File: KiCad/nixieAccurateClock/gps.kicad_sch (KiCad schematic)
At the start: 3 parts

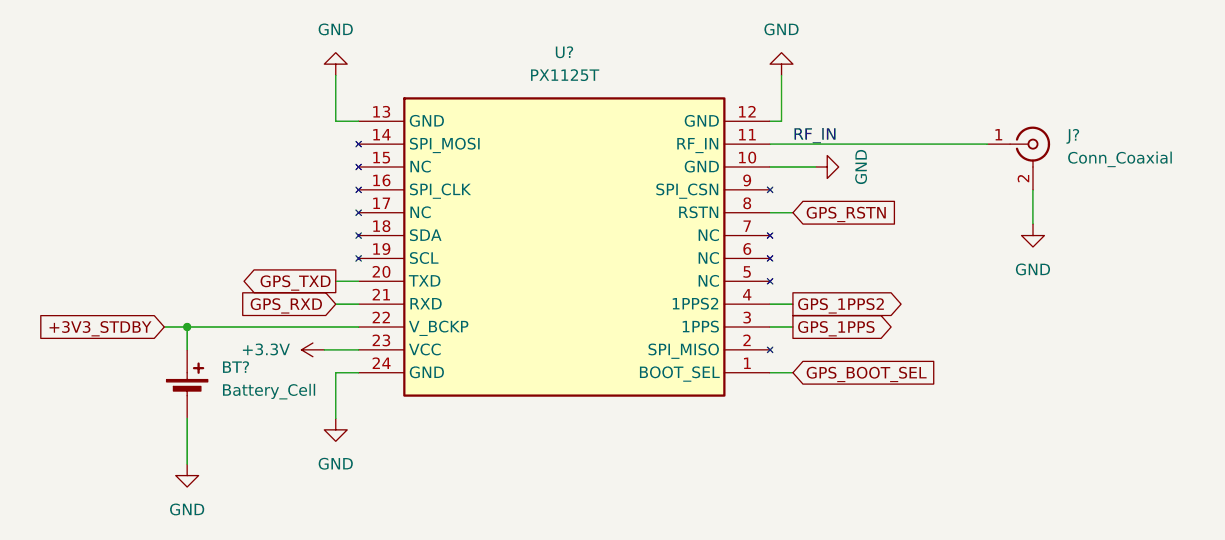
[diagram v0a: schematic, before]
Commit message: Signal condition shunt signal
Textbook reference and LTSpice simulation for receipts.

I attempted a differential amplifier based solution but I failed to get it to work.  If it did work it would require more components and likely give little additional benefit.

ADC implementation WIP.
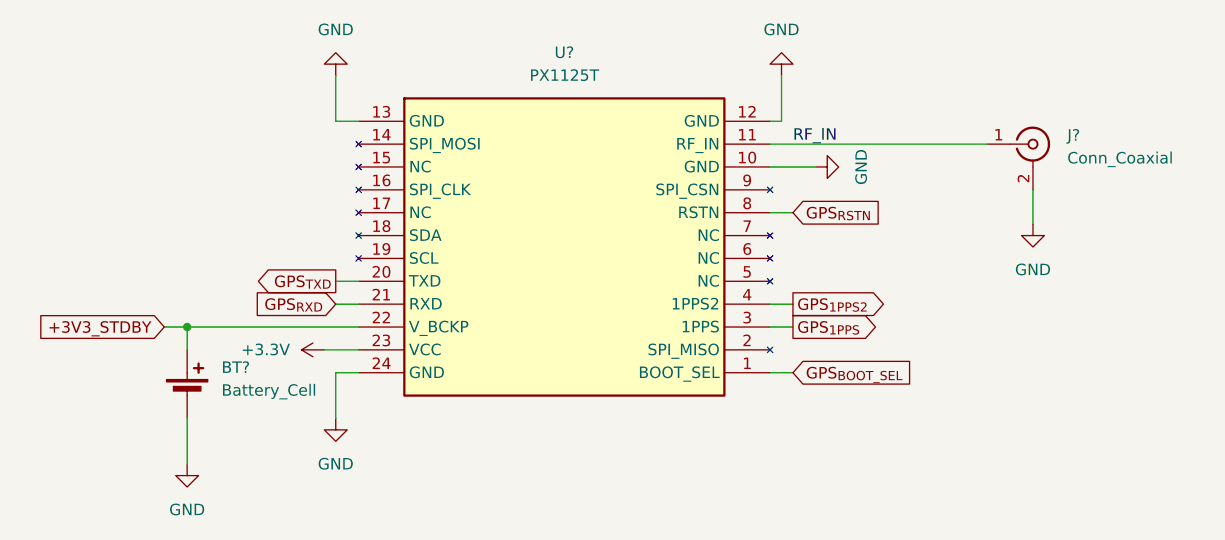
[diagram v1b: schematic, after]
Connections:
- net GPS_1PPS renamed GPS_{1PPS}
- net GPS_1PPS2 renamed GPS_{1PPS2}
- net GPS_BOOT_SEL renamed GPS_{BOOT_SEL}
- net GPS_RSTN renamed GPS_{RSTN}
- net GPS_RXD renamed GPS_{RXD}
- net GPS_TXD renamed GPS_{TXD}
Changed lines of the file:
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@@
     (effects (font (size 1.27 1.27)) (justify left bottom))
   )
-  (global_label "GPS_RSTN" (shape input) (at 157.48 97.79 0) (fields_autoplaced)
+  (global_label "GPS_{RSTN}" (shape input) (at 157.48 97.79 0) (fields_autoplaced)
     (effects (font (size 1.27 1.27)) (justify left))
-    (property "Intersheetrefs" "${INTERSHEET_REFS}" (at 169.9599 97.79 0)
+    (property "Intersheetrefs" "${INTERSHEET_REFS}" (at 168.0876 97.79 0)
       (effects (font (size 1.27 1.27)) (justify left) hide)
     )
   )
-  (global_label "GPS_TXD" (shape output) (at 106.68 105.41 180) (fields_autoplaced)
+  (global_label "GPS_{TXD}" (shape output) (at 106.68 105.41 180) (fields_autoplaced)
     (effects (font (size 1.27 1.27)) (justify right))
-    (property "Intersheetrefs" "${INTERSHEET_REFS}" (at 95.5306 105.41 0)
+    (property "Intersheetrefs" "${INTERSHEET_REFS}" (at 97.1368 105.41 0)
       (effects (font (size 1.27 1.27)) (justify right) hide)
     )
@@
     )
   )
-  (global_label "GPS_BOOT_SEL" (shape input) (at 157.48 115.57 0) (fields_autoplaced)
+  (global_label "GPS_{BOOT_SEL}" (shape input) (at 157.48 115.57 0) (fields_autoplaced)
     (effects (font (size 1.27 1.27)) (justify left))
-    (property "Intersheetrefs" "${INTERSHEET_REFS}" (at 174.4351 115.57 0)
+    (property "Intersheetrefs" "${INTERSHEET_REFS}" (at 171.6678 115.57 0)
       (effects (font (size 1.27 1.27)) (justify left) hide)
     )
   )
-  (global_label "GPS_1PPS2" (shape output) (at 157.48 107.95 0) (fields_autoplaced)
+  (global_label "GPS_{1PPS2}" (shape output) (at 157.48 107.95 0) (fields_autoplaced)
     (effects (font (size 1.27 1.27)) (justify left))
-    (property "Intersheetrefs" "${INTERSHEET_REFS}" (at 171.3508 107.95 0)
+    (property "Intersheetrefs" "${INTERSHEET_REFS}" (at 169.2003 107.95 0)
       (effects (font (size 1.27 1.27)) (justify left) hide)
     )
   )
-  (global_label "GPS_1PPS" (shape output) (at 157.48 110.49 0) (fields_autoplaced)
+  (global_label "GPS_{1PPS}" (shape output) (at 157.48 110.49 0) (fields_autoplaced)
     (effects (font (size 1.27 1.27)) (justify left))
-    (property "Intersheetrefs" "${INTERSHEET_REFS}" (at 170.1413 110.49 0)
+    (property "Intersheetrefs" "${INTERSHEET_REFS}" (at 168.2327 110.49 0)
       (effects (font (size 1.27 1.27)) (justify left) hide)
     )
   )
-  (global_label "GPS_RXD" (shape input) (at 106.68 107.95 180) (fields_autoplaced)
+  (global_label "GPS_{RXD}" (shape input) (at 106.68 107.95 180) (fields_autoplaced)
     (effects (font (size 1.27 1.27)) (justify right))
-    (property "Intersheetrefs" "${INTERSHEET_REFS}" (at 95.2282 107.95 0)
+    (property "Intersheetrefs" "${INTERSHEET_REFS}" (at 96.8949 107.95 0)
       (effects (font (size 1.27 1.27)) (justify right) hide)
     )
@@
         )
         (path "/55aab698-7558-4fe2-95ad-faa6da60ef89/9610945c-9df3-4d66-a574-d19433fdc707"
+          (reference "#PWR022") (unit 1)
+        )
+      )
+    )
+  )
+  (symbol (lib_id "power:GND") (at 90.17 125.73 0) (mirror y) (unit 1)
+    (in_bom yes) (on_board yes) (dnp no)
+    (property "Reference" "#PWR?" (at 90.17 132.08 0)
+      (effects (font (size 1.27 1.27)) hide)
+    )
+    (property "Value" "GND" (at 90.17 130.81 0)
+      (effects (font (size 1.27 1.27)))
+    )
+    (property "Footprint" "" (at 90.17 125.73 0)
+      (effects (font (size 1.27 1.27)) hide)
+    )
+    (property "Datasheet" "" (at 90.17 125.73 0)
+      (effects (font (size 1.27 1.27)) hide)
+    )
+    (pin "1")
+    (instances
+      (project "nixieAccurateClock"
+        (path "/55aab698-7558-4fe2-95ad-faa6da60ef89"
+          (reference "#PWR?") (unit 1)
+        )
+        (path "/55aab698-7558-4fe2-95ad-faa6da60ef89/9610945c-9df3-4d66-a574-d19433fdc707"
+          (reference "#PWR017") (unit 1)
+        )
+      )
+    )
+  )
+  (symbol (lib_id "power:GND") (at 184.15 99.06 0) (mirror y) (unit 1)
+    (in_bom yes) (on_board yes) (dnp no)
+    (property "Reference" "#PWR?" (at 184.15 105.41 0)
+      (effects (font (size 1.27 1.27)) hide)
+    )
+    (property "Value" "GND" (at 184.15 104.14 0)
+      (effects (font (size 1.27 1.27)))
+    )
+    (property "Footprint" "" (at 184.15 99.06 0)
+      (effects (font (size 1.27 1.27)) hide)
+    )
+    (property "Datasheet" "" (at 184.15 99.06 0)
+      (effects (font (size 1.27 1.27)) hide)
+    )
+    (pin "1")
+    (instances
+      (project "nixieAccurateClock"
+        (path "/55aab698-7558-4fe2-95ad-faa6da60ef89"
+          (reference "#PWR?") (unit 1)
+        )
+        (path "/55aab698-7558-4fe2-95ad-faa6da60ef89/9610945c-9df3-4d66-a574-d19433fdc707"
           (reference "#PWR023") (unit 1)
         )
@@
     )
   )
-  (symbol (lib_id "power:GND") (at 90.17 125.73 0) (mirror y) (unit 1)
-    (in_bom yes) (on_board yes) (dnp no)
-    (property "Reference" "#PWR?" (at 90.17 132.08 0)
-      (effects (font (size 1.27 1.27)) hide)
-    )
-    (property "Value" "GND" (at 90.17 130.81 0)
-      (effects (font (size 1.27 1.27)))
-    )
-    (property "Footprint" "" (at 90.17 125.73 0)
-      (effects (font (size 1.27 1.27)) hide)
-    )
-    (property "Datasheet" "" (at 90.17 125.73 0)
-      (effects (font (size 1.27 1.27)) hide)
-    )
-    (pin "1")
-    (instances
-      (project "nixieAccurateClock"
-        (path "/55aab698-7558-4fe2-95ad-faa6da60ef89"
-          (reference "#PWR?") (unit 1)
-        )
-        (path "/55aab698-7558-4fe2-95ad-faa6da60ef89/9610945c-9df3-4d66-a574-d19433fdc707"
-          (reference "#PWR018") (unit 1)
-        )
-      )
-    )
-  )
-  (symbol (lib_id "power:GND") (at 184.15 99.06 0) (mirror y) (unit 1)
-    (in_bom yes) (on_board yes) (dnp no)
-    (property "Reference" "#PWR?" (at 184.15 105.41 0)
-      (effects (font (size 1.27 1.27)) hide)
-    )
-    (property "Value" "GND" (at 184.15 104.14 0)
-      (effects (font (size 1.27 1.27)))
-    )
-    (property "Footprint" "" (at 184.15 99.06 0)
-      (effects (font (size 1.27 1.27)) hide)
-    )
-    (property "Datasheet" "" (at 184.15 99.06 0)
-      (effects (font (size 1.27 1.27)) hide)
-    )
-    (pin "1")
-    (instances
-      (project "nixieAccurateClock"
-        (path "/55aab698-7558-4fe2-95ad-faa6da60ef89"
-          (reference "#PWR?") (unit 1)
-        )
-        (path "/55aab698-7558-4fe2-95ad-faa6da60ef89/9610945c-9df3-4d66-a574-d19433fdc707"
-          (reference "#PWR024") (unit 1)
-        )
-      )
-    )
-  )
   (symbol (lib_id "power:GND") (at 106.68 82.55 180) (unit 1)
     (in_bom yes) (on_board yes) (dnp no)
@@
         )
         (path "/55aab698-7558-4fe2-95ad-faa6da60ef89/9610945c-9df3-4d66-a574-d19433fdc707"
-          (reference "#PWR020") (unit 1)
+          (reference "#PWR019") (unit 1)
         )
       )
@@
         )
         (path "/55aab698-7558-4fe2-95ad-faa6da60ef89/9610945c-9df3-4d66-a574-d19433fdc707"
-          (reference "#PWR019") (unit 1)
+          (reference "#PWR018") (unit 1)
         )
       )
@@
         )
         (path "/55aab698-7558-4fe2-95ad-faa6da60ef89/9610945c-9df3-4d66-a574-d19433fdc707"
-          (reference "#PWR022") (unit 1)
+          (reference "#PWR021") (unit 1)
         )
       )
@@
         )
         (path "/55aab698-7558-4fe2-95ad-faa6da60ef89/9610945c-9df3-4d66-a574-d19433fdc707"
-          (reference "#PWR021") (unit 1)
-        )
-      )
+          (reference "#PWR020") (unit 1)
+        )
+      )
